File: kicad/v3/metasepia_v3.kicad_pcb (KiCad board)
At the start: 2 copper layers, 227.9 x 132.7 mm, 66 parts

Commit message: create slider switch, battery pad, add to v3
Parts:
- added BT1: Battery_Cell, frequent:bat, F.Cu at (170.4, 151.0)
- added BT1: Battery_Cell, frequent:bat, F.Cu at (230.3, 151.0)
- moved REF** 25.0 mm to (200.3, 116.0)
- moved D16 24.9 mm to (288.3, 106.1)
- moved D2 24.9 mm to (101.5, 76.9)
- moved S8 24.9 mm to (152.4, 74.7)
- moved _3 24.9 mm to (150.6, 168.9)
- moved _4 24.9 mm to (250.1, 168.9)
- moved D30 24.9 mm to (249.4, 180.0)
- moved S16 24.9 mm to (286.7, 102.5)
- moved D10 24.9 mm to (152.8, 113.5)
- moved D13 24.9 mm to (173.1, 117.2)
- moved D21 24.9 mm to (250.3, 78.1)
- moved D22 24.9 mm to (258.2, 129.5)
- moved D26 24.9 mm to (227.6, 117.2)
- moved S14 24.9 mm to (303.6, 91.3)
- moved S26 24.9 mm to (225.4, 113.8)
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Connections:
- REF** pad 3: (no net) -> BAT_POS
- REF** pad 6: (no net) -> BAT_POS
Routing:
- net BAT_NEG: track 0.00 -> 133.3 mm
- net (no net): track 0.00 -> 124.0 mm, vias 0 -> 1
- net BAT_POS: track 0.00 -> 21.1 mm, vias 0 -> 1
- net P8: track 235.8 -> 249.8 mm
- net P3: track 265.1 -> 263.8 mm
- net GND: vias 8 -> 12

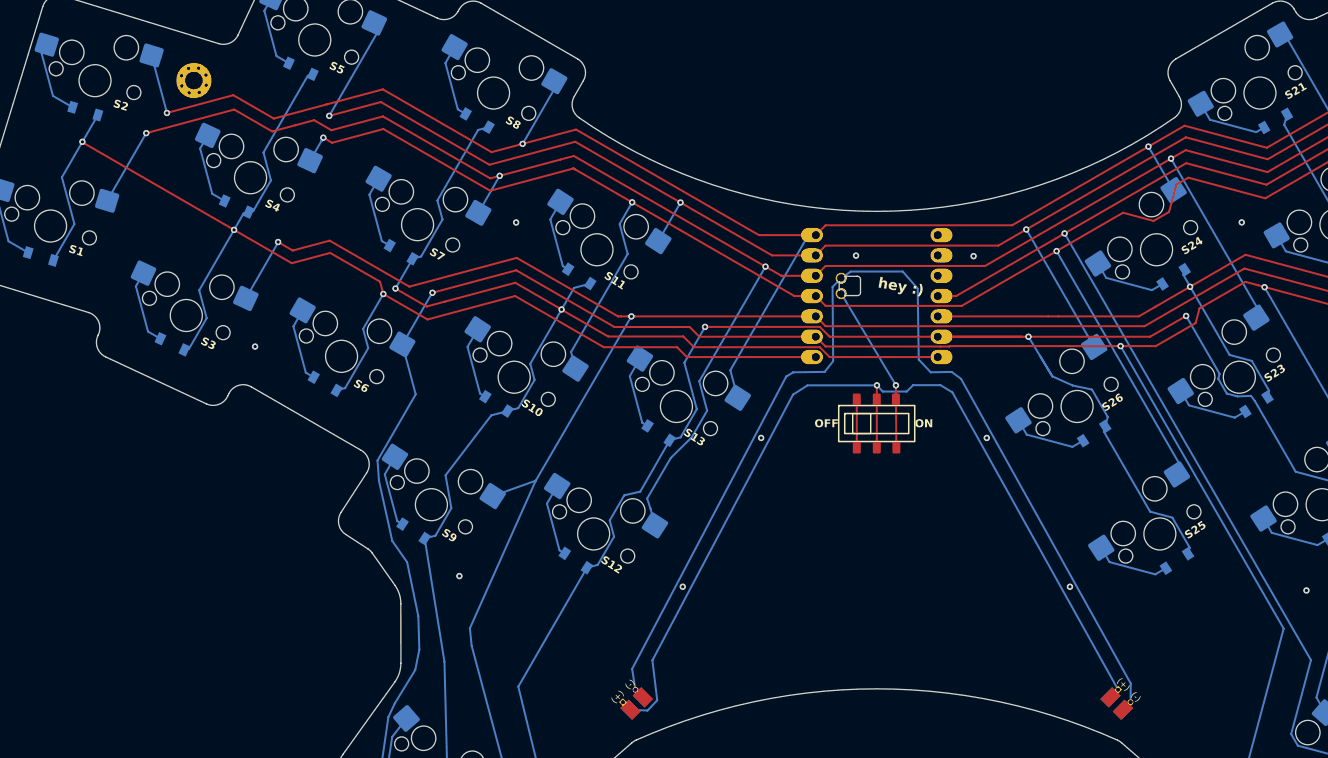
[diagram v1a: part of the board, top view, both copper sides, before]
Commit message: update
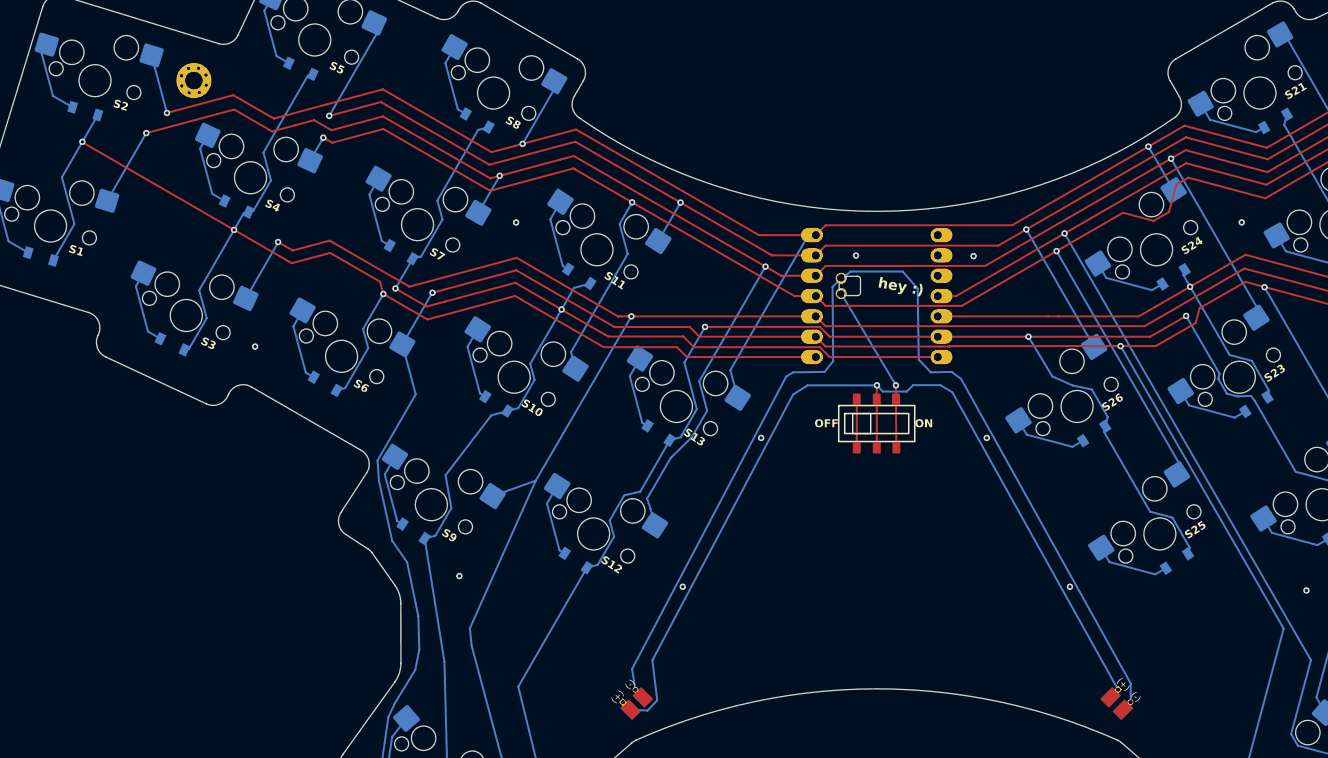
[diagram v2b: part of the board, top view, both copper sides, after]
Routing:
- net P8: track 249.8 -> 236.2 mm
